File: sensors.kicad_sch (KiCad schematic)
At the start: 53 parts, among them J1 1-4, J2 5-8, U1 ADG707, U2 OPA2340, U3 OPA2340

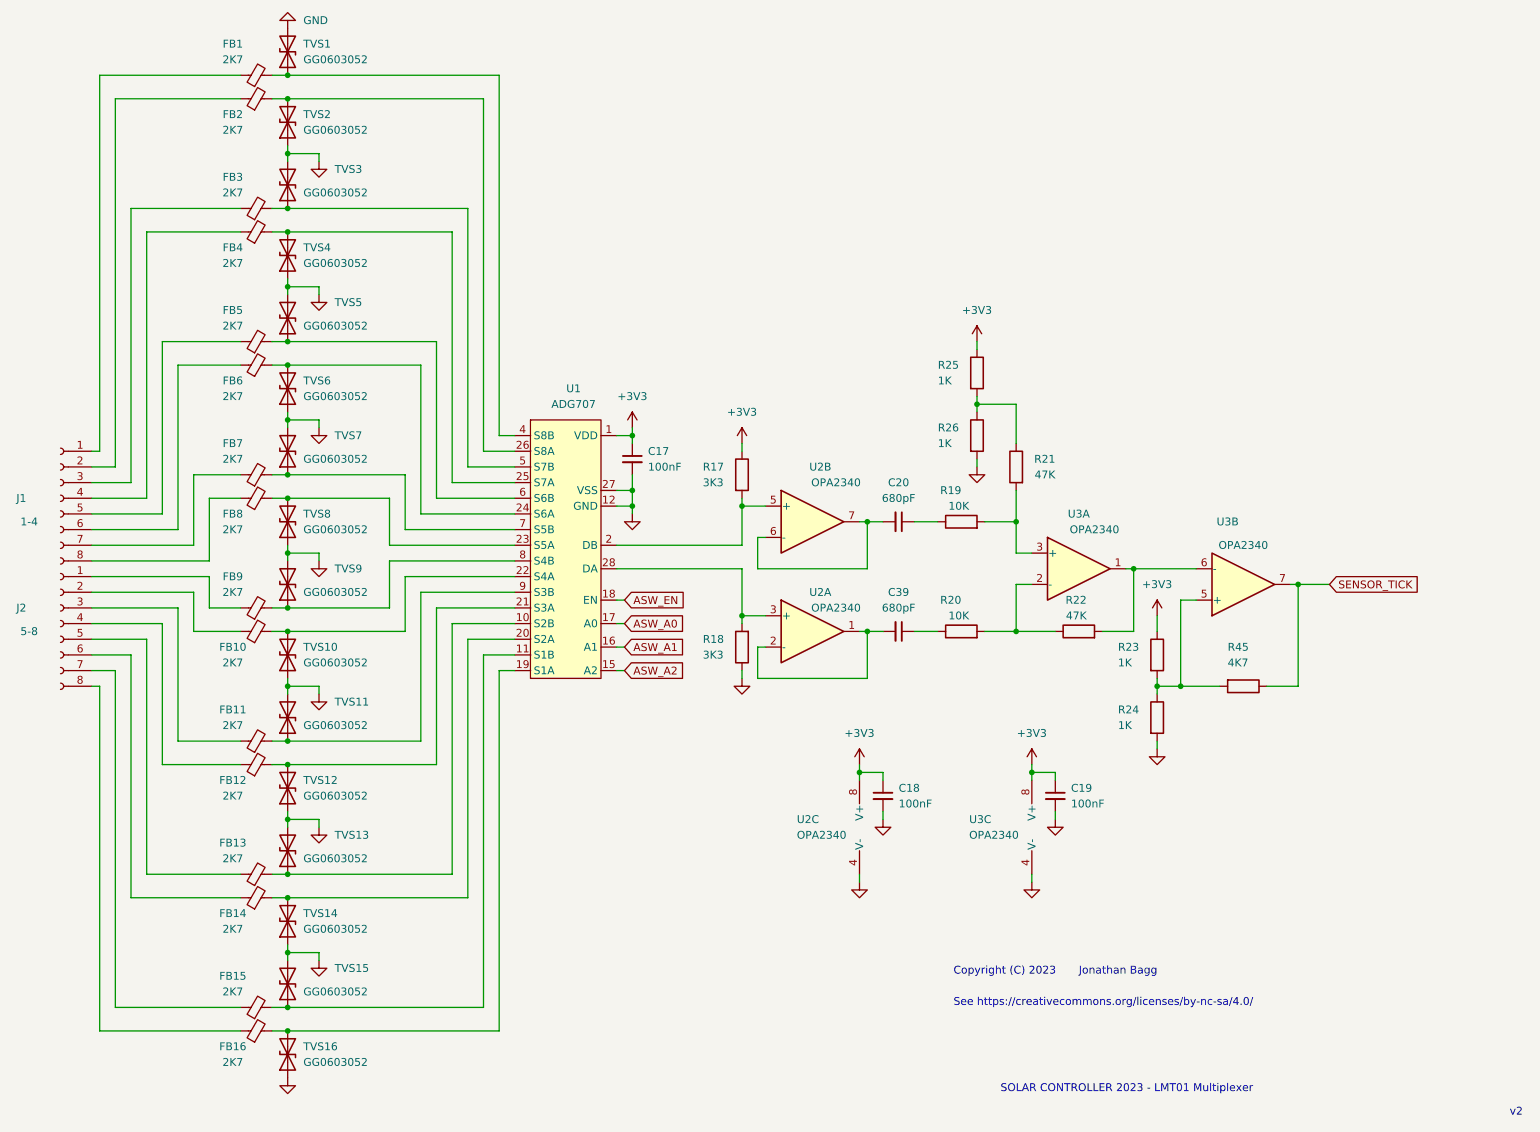
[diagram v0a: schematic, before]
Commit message: generate gerbers
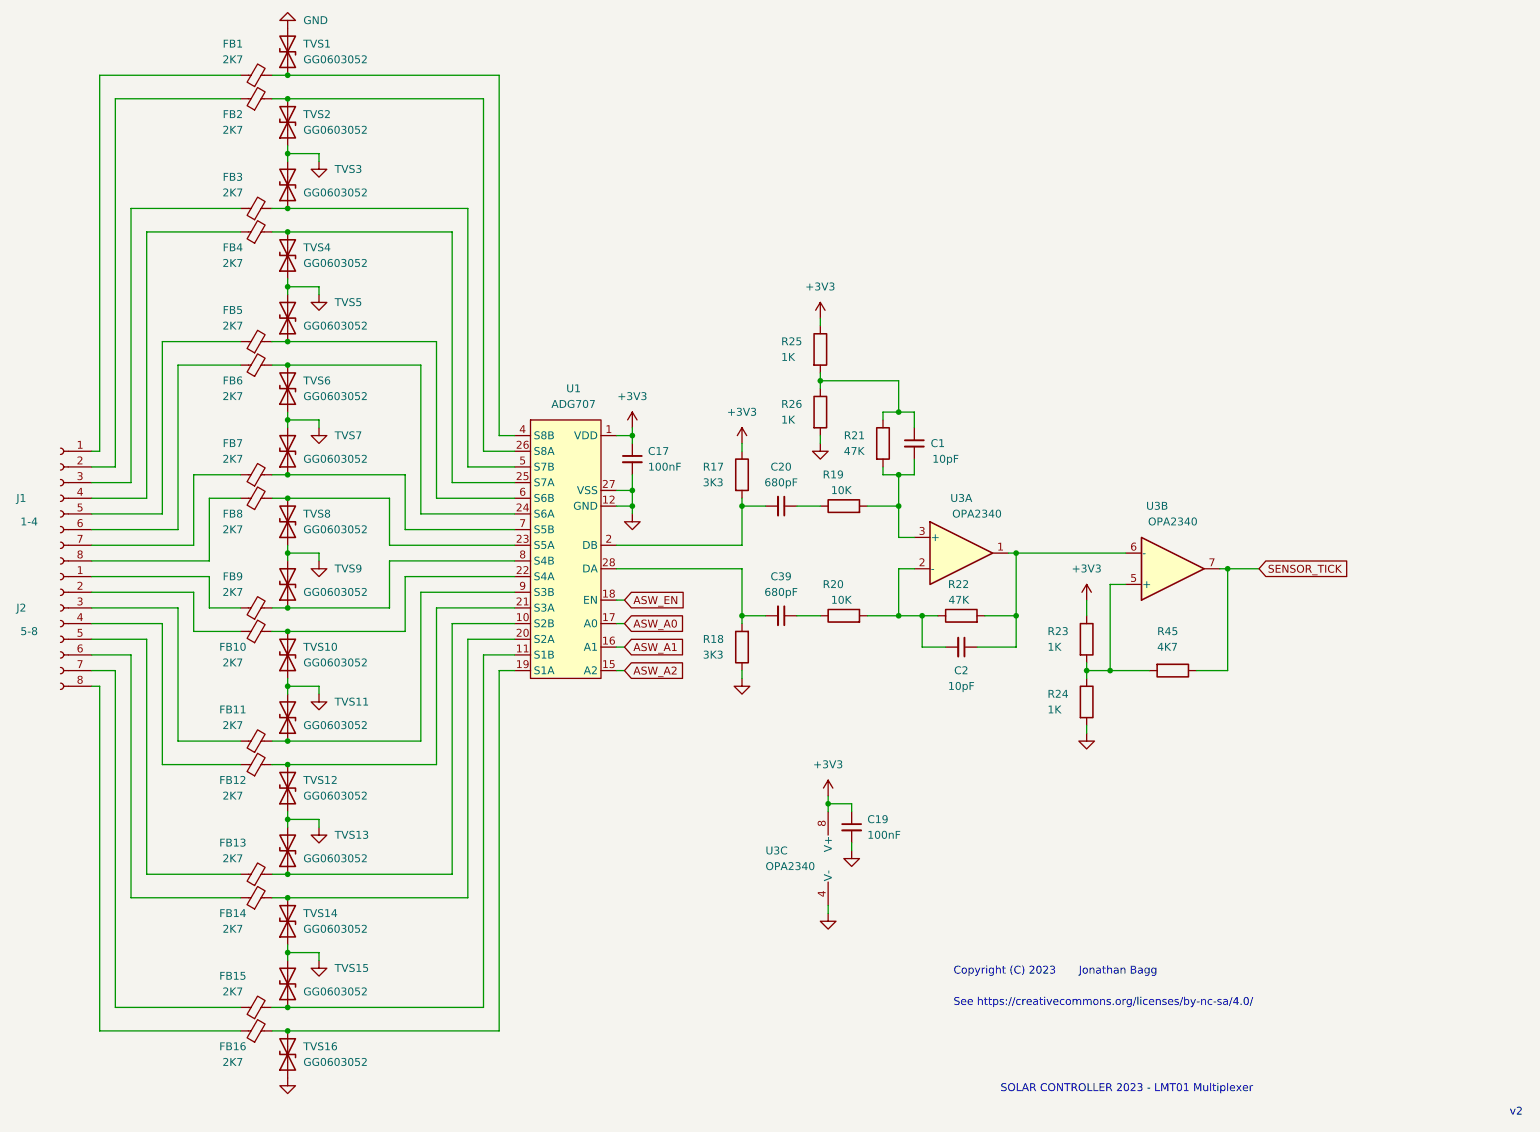
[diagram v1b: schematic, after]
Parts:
- removed C18: 100nF, Capacitor_SMD:C_0603_1608Metric_Pad1.08x0.95mm_HandSolder, symbol Device:C_Small
- removed U2: OPA2340, Package_SO:SOP-8_3.9x4.9mm_P1.27mm, symbol Amplifier_Operational:OPA2340
- added C1, C2: 10pF, Capacitor_SMD:C_0603_1608Metric_Pad1.08x0.95mm_HandSolder, symbol Device:C_Small
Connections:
- net at C39.2: now also R18.2, U1.28 (DA)
- net at R19.2, R21.2, U3.3 (+): now also C1.2
- net at R20.2, R22.1, U3.2 (-): now also C2.2
- net at R22.2, U3.1, U3.6 (-): now also C2.1
- net at R21.1, R25.2, R26.1: now also C1.1
- net at R17.2, U1.2 (DB): now also C20.2
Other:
- moved on the sheet: C19, C20, C39, R19, R20, R21, R22, R23, R24, R25, R26, R45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
